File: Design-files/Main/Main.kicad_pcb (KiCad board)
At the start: 2 copper layers, 25 parts, among them J1 USB_B_Micro, J2 Conn_01x02_Pin, J3 Conn_01x24_Pin, J4 Conn_01x24_Socket, J5 Conn_01x24_Socket, J6 Conn_01x24_Pin, J7 Conn_01x10_Pin, U1 CH340C, U2 CAT24C256, U3 HT75xx-1-SOT89, U4 LTC4054ES5-4.2, U6 TPS2115A-Q1

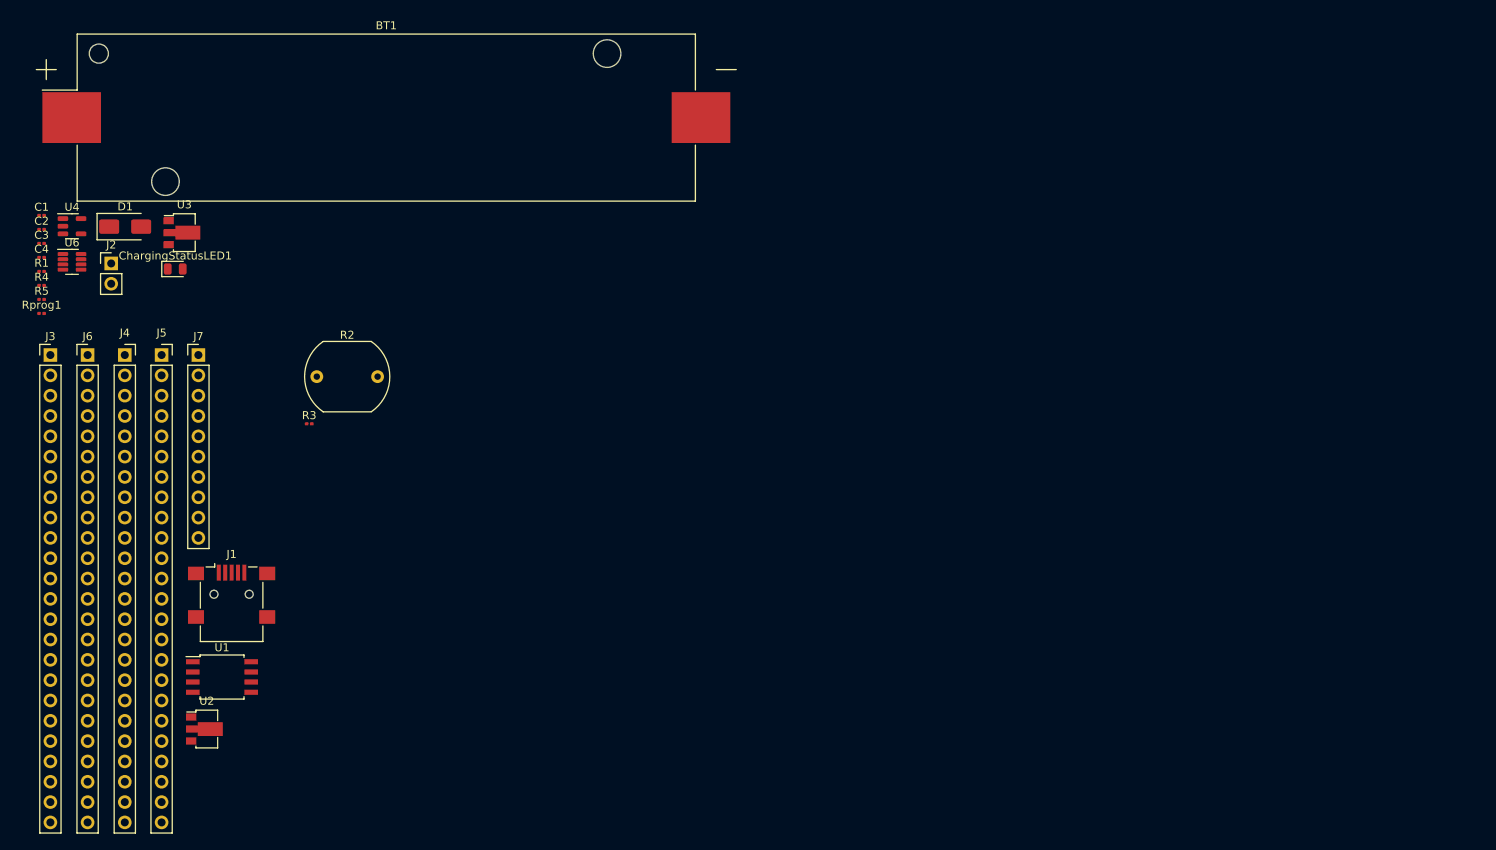
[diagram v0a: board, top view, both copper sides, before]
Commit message: changes
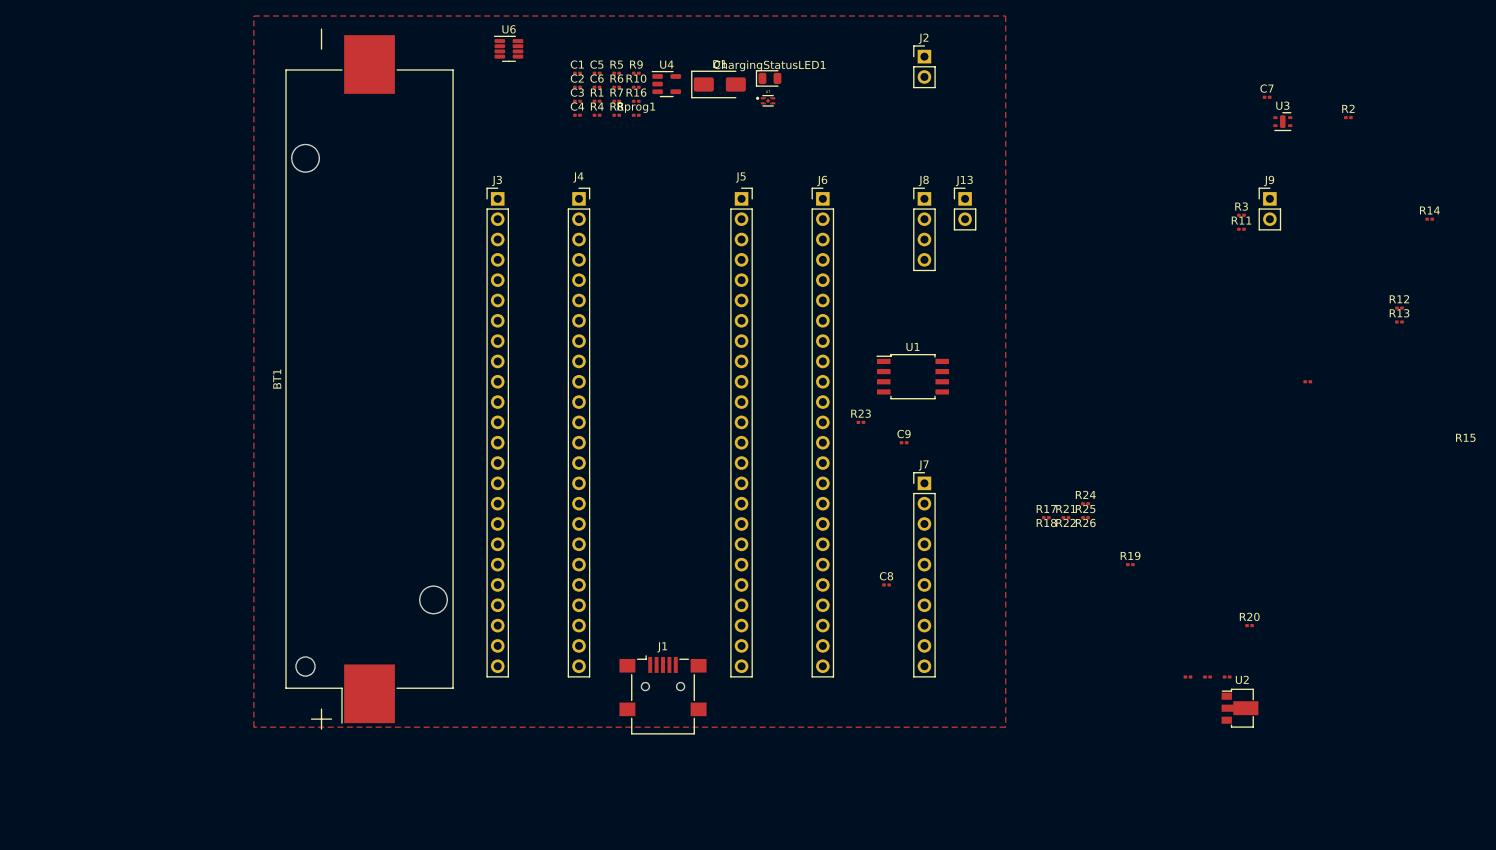
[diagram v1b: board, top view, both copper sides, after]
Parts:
- added C5: 1 uF, Capacitor_SMD:C_0201_0603Metric, F.Cu at (136.9, 52.9)
- added C6: 1 uF, Capacitor_SMD:C_0201_0603Metric, F.Cu at (136.9, 54.6)
- added C7: 10 uF, Capacitor_SMD:C_0201_0603Metric, F.Cu at (220.6, 55.9)
- added C8: 0.1uF, Capacitor_SMD:C_0201_0603Metric, F.Cu at (173.1, 116.8)
- added C9: 0.1uF, Capacitor_SMD:C_0201_0603Metric, F.Cu at (175.3, 99.1)
- added J13: Conn_01x02_Pin, Connector_PinHeader_2.54mm:PinHeader_1x02_P2.54mm_Vertical, F.Cu at (182.9, 68.6)
- added J8: Conn_01x04_Pin, Connector_PinHeader_2.54mm:PinHeader_1x04_P2.54mm_Vertical, F.Cu at (177.8, 68.6)
- added J9: Conn_01x02_Pin, Connector_PinHeader_2.54mm:PinHeader_1x02_P2.54mm_Vertical, F.Cu at (221.0, 68.6)
- added R10: 0, Resistor_SMD:R_0201_0603Metric, F.Cu at (141.8, 54.6)
- added R11: 10000, Resistor_SMD:R_0201_0603Metric, F.Cu at (217.4, 72.4)
- added R12: 10000, Resistor_SMD:R_0201_0603Metric, F.Cu at (237.2, 82.2)
- added R13: 0, Resistor_SMD:R_0201_0603Metric, F.Cu at (237.2, 84.0)
- added R14: 0, Resistor_SMD:R_0201_0603Metric, F.Cu at (241.0, 71.1)
- added R15: 0, Resistor_SMD:R_0201_0603Metric, F.Cu at (225.7, 91.4)
- added R16: 0, Resistor_SMD:R_0201_0603Metric, F.Cu at (141.8, 56.4)
- added R17: 0, Resistor_SMD:R_0201_0603Metric, F.Cu at (193.0, 108.4)
- added R18: 0, Resistor_SMD:R_0201_0603Metric, F.Cu at (210.7, 128.3)
- added R19: 4700, Resistor_SMD:R_0201_0603Metric, F.Cu at (203.5, 114.3)
- added R20: 4700, Resistor_SMD:R_0201_0603Metric, F.Cu at (218.4, 121.9)
- added R21: 0, Resistor_SMD:R_0201_0603Metric, F.Cu at (195.5, 108.4)
- added R22: 0, Resistor_SMD:R_0201_0603Metric, F.Cu at (213.2, 128.3)
- added R23: 0, Resistor_SMD:R_0201_0603Metric, F.Cu at (169.9, 96.5)
- added R24: 0, Resistor_SMD:R_0201_0603Metric, F.Cu at (197.9, 106.7)
- added R25: 0, Resistor_SMD:R_0201_0603Metric, F.Cu at (197.9, 108.4)
- added R26: 0, Resistor_SMD:R_0201_0603Metric, F.Cu at (215.6, 128.3)
- added R6: 0, Resistor_SMD:R_0201_0603Metric, F.Cu at (139.3, 54.6)
- added R7: 0, Resistor_SMD:R_0201_0603Metric, F.Cu at (139.3, 56.4)
- added R8: 0, Resistor_SMD:R_0201_0603Metric, F.Cu at (139.3, 58.1)
- added R9: 0, Resistor_SMD:R_0201_0603Metric, F.Cu at (141.8, 52.9)
- added U7: RT9073A, REG_RT9080-33GQZ:REG_RT9080-33GQZ, F.Cu at (158.3, 56.3)
- J2: value Conn_01x02_Pin -> Battery Jumper
- R2: value LDR03 -> 100K; footprint OptoDevice:R_LDR_10x8.5mm_P7.6mm_Vertical -> Resistor_SMD:R_0201_0603Metric
- R3: value 150K -> 100K
- Rprog1: value 2000 -> 1000
- U3: value HT75xx-1-SOT89 -> SHTC3; footprint Package_TO_SOT_SMD:SOT-89-3 -> Sensor_Humidity:Sensirion_DFN-4-1EP_2x2mm_P1mm_EP0.7x1.6mm
- moved U3 138.0 mm to (222.6, 58.9)
- moved R2 133.0 mm to (230.8, 58.4)
- moved U2 129.5 mm to (217.5, 132.2)
- moved R3 119.4 mm to (217.4, 70.6)
- moved J2 104.9 mm to (177.8, 50.8)
- moved U1 94.2 mm to (176.4, 90.8)
- moved J6 94.0 mm to (165.1, 68.6)
- moved J7 92.2 mm to (177.8, 104.1)
- moved Rprog1 78.4 mm to (141.8, 58.1)
- moved ChargingStatusLED1 78.1 mm to (158.5, 53.5)
- moved R5 77.2 mm to (139.3, 52.9)
- moved U4 76.4 mm to (145.6, 54.2)
- moved D1 76.4 mm to (152.2, 54.3)
- moved J5 75.1 mm to (154.9, 68.6)
- moved R1 72.6 mm to (136.9, 56.4)
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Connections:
- net AnalogueSensorOut renamed /BatterySense
- net DigitalSensorSCL renamed /DigitalSensorSCL
- net DigitalSensorSDA renamed /DigitalSensorSDA
- net EEPROMSCL renamed /Interfacing/EEPROMSCL
- net EEPROMSDA renamed /Interfacing/EEPROMSDA
- C2 pad 2: USB 5V -> Net-(ChargingStatusLED1-A)
- C3 pad 1: Battery Input Polarity Protection -> /Power Module/Battery Input Polarity Protection
- C4 pad 2: USB 5V -> Net-(U6-IN1)
- ChargingStatusLED1 pad 2: USB 5V -> Net-(ChargingStatusLED1-A)
- D1 pad 1: Battery Input Polarity Protection -> Net-(D1-K)
- J1 pad 1: USB 5V -> /USB 5V
- J1 pad 2: USB D- -> /Interfacing/USB D-
- J1 pad 3: USB D+ -> /Interfacing/USB D+
- J3 pad 11: USB 5V -> /USB 5V
- J3 pad 24: Regulated 3v3 -> /Regulated 3v3
- J4 pad 11: USB 5V -> /USB 5V
- J4 pad 24: Regulated 3v3 -> /Regulated 3v3
- J5 pad 6: USART_TX -> /Interfacing/USART_TX
- J5 pad 7: USART_RX -> /Interfacing/USART_RX
- J6 pad 6: USART_TX -> /Interfacing/USART_TX
- J6 pad 7: USART_RX -> /Interfacing/USART_RX
- J7 pad 1: Regulated 3v3 -> /Regulated 3v3
- J7 pad 7: USB 5V -> /USB 5V
- J7 pad 8: USART_TX -> /Interfacing/USART_TX
- J7 pad 9: USART_RX -> /Interfacing/USART_RX
- R3 pad 1: Regulated 3v3 -> Battery
- R4 pad 2: Switched Power -> Net-(U6-OUT)
- U1 pad 2: USART_RX -> Net-(U1-TXD)
- U1 pad 3: USART_TX -> Net-(U1-RXD)
- U1 pad 4: unconnected-(U1-V3-Pad4) -> Net-(U1-V3)
- U1 pad 5: USB D+ -> Net-(U1-UD+)
- U1 pad 6: USB D- -> Net-(U1-UD-)
- U3 pad 1: GND -> Net-(U3-VDD)
- U3 pad 2: Switched Power -> Net-(U3-SCL)
- U3 pad 3: Regulated 3v3 -> Net-(U3-SDA)
- U4 pad 3: Battery -> Net-(U4-BAT)
- U4 pad 4: USB 5V -> Net-(ChargingStatusLED1-A)
- U6 pad 6: Battery Input Polarity Protection -> /Power Module/Battery Input Polarity Protection
- U6 pad 7: Switched Power -> Net-(U6-OUT)
- U6 pad 8: USB 5V -> Net-(U6-IN1)
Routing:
- added copper zone on F.Cu, net GND
